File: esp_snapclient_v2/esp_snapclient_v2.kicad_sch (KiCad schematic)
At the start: 13 parts, among them SW1 SW_Push, SW2 SW_Push, U1 ESP32-WROVER-E, U2 MAX98357A, U3 MAX98357A

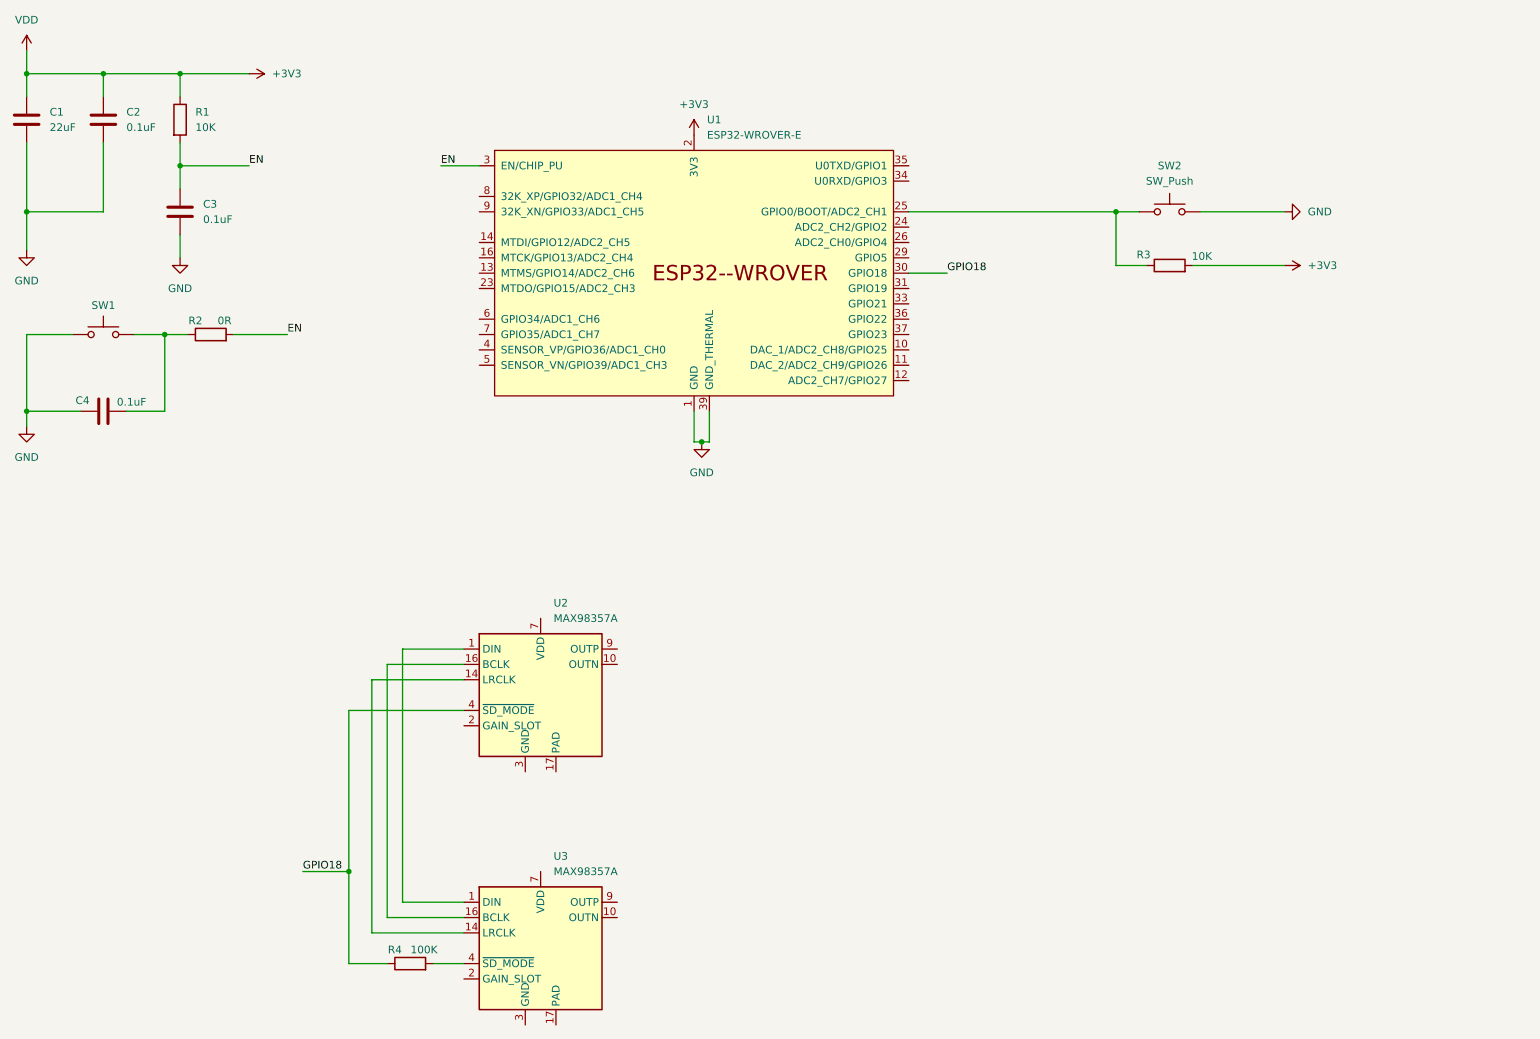
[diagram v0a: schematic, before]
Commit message: feat: up
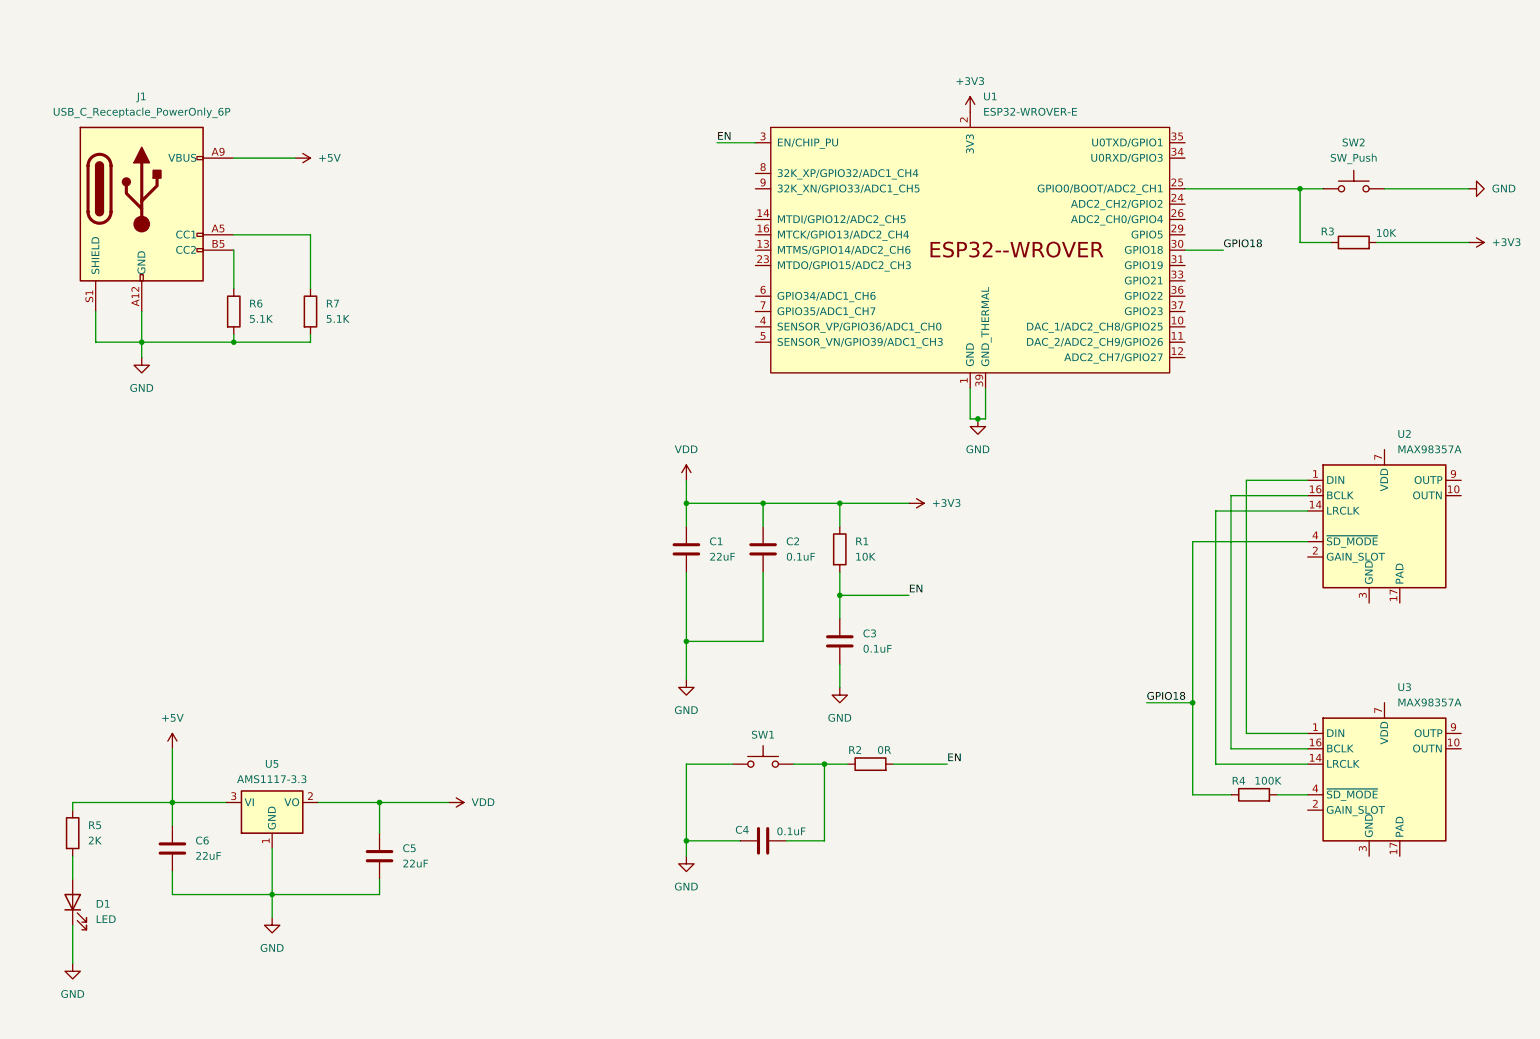
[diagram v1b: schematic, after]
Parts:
- added C5, C6: 22uF, Capacitor_SMD:C_0805_2012Metric, symbol Device:C
- added D1: LED, symbol Device:LED
- added J1: USB_C_Receptacle_PowerOnly_6P, symbol Connector:USB_C_Receptacle_PowerOnly_6P
- added R5: 2K, Resistor_SMD:R_0805_2012Metric, symbol Device:R
- added R6, R7: 5.1K, Resistor_SMD:R_0805_2012Metric, symbol Device:R
- added U5: AMS1117-3.3, Package_TO_SOT_SMD:SOT-223-3_TabPin2, symbol Regulator_Linear:AMS1117-3.3
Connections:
- net +3V3: now also C5.1, U5.2 (VO)
- net GND: now also C5.2, C6.2, D1.1 (K), J1.A12 (GND), J1.B12 (GND), J1.S1 (SHIELD), R6.2, R7.2, U5.1 (GND)
- new net: J1.A5 (CC1), R7.1
- new net: D1.2 (A), R5.2
- new net: J1.B5 (CC2), R6.1
- new net +5V: C6.1, J1.A9 (VBUS), J1.B9 (VBUS), R5.1, U5.3 (VI)
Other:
- moved on the sheet: C1, C2, C3, C4, R1, R2, R3, R4, SW1, SW2, U1, U2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
